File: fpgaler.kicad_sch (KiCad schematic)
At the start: 118 parts, among them J1 USB_C_Receptacle_USB2.0, J3 JTAG, J4 FTDI_RST, J5 VGA, J6 DB9 Expander 1, J7 DB9 Expander 0, Q2 BC817, SW1 ROT, SW2 ROT1, SW3 K1, SW4 K2, SW5 PROGRAM, SW6 K3, SW7 FPGA GSRN, SW8 K4

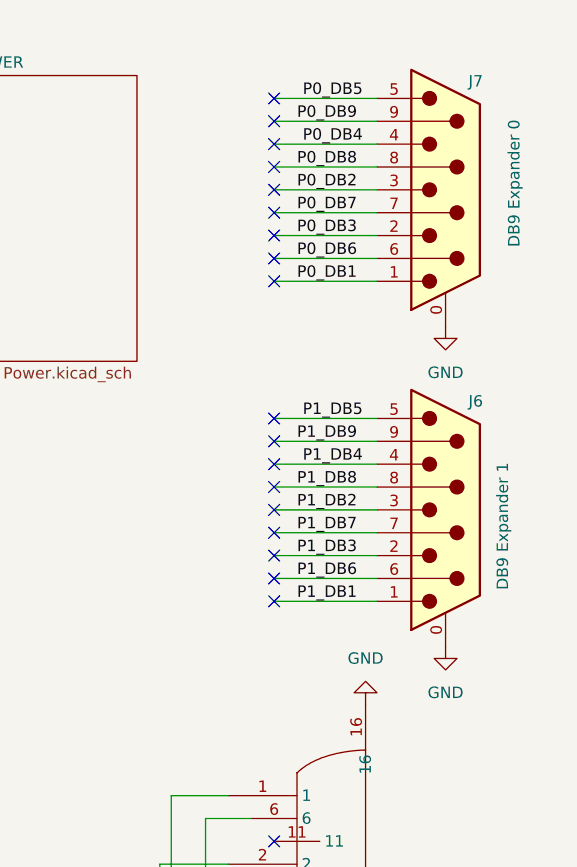
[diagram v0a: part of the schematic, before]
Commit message: Complete
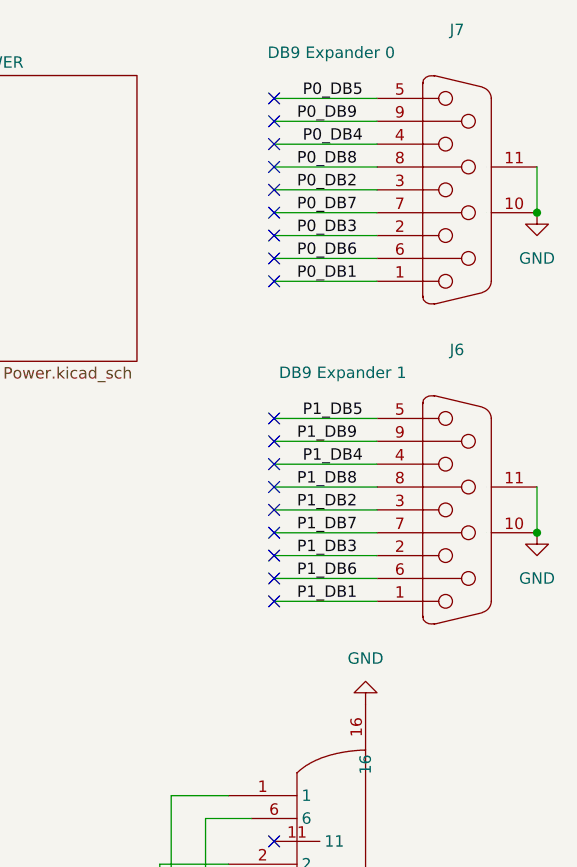
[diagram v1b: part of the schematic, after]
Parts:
- removed J6: DB9 Expander 1, Connector_Dsub:DSUB-9_Pins_Horizontal_P2.77x2.84mm_EdgePinOffset4.94mm_Housed_MountingHolesOffset4.94mm, symbol Connector:DE9_Pins_MountingHoles
- removed J7: DB9 Expander 0, Connector_Dsub:DSUB-9_Pins_Horizontal_P2.77x2.84mm_EdgePinOffset4.94mm_Housed_MountingHolesOffset4.94mm, symbol Connector:DE9_Pins_MountingHoles
- added J6: DB9 Expander 1, EasyEDA_Lib:DSUB-TH_DMR-9P, symbol EasyEDA_Lib:DMR-9P
- added J7: DB9 Expander 0, EasyEDA_Lib:DSUB-TH_DMR-9P, symbol EasyEDA_Lib:DMR-9P
- J1: PN USB4105-GF-A -> (none); PN_1 C167321 -> C2765186
- TP1, TP20: value TestPoint -> 3.3V
- TP19, TP23: value TestPoint -> GND
- TP24, TP25: value TestPoint -> 2.5V
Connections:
- net GND: now also J6.10 (MH1), J6.11 (MH2), J7.10 (MH1), J7.11 (MH2)
- net P0_DB1: now also J7.1
- net P0_DB2: now also J7.3
- net P0_DB3: now also J7.2
- net P0_DB4: now also J7.4
- net P0_DB5: now also J7.5
- net P0_DB6: now also J7.6
- net P0_DB7: now also J7.7
- net P0_DB8: now also J7.8
- net P0_DB9: now also J7.9
- net P1_DB1: now also J6.1
- net P1_DB2: now also J6.3
- net P1_DB3: now also J6.2
- net P1_DB4: now also J6.4
- net P1_DB5: now also J6.5
- net P1_DB6: now also J6.6
- net P1_DB7: now also J6.7
- net P1_DB8: now also J6.8
- net P1_DB9: now also J6.9
